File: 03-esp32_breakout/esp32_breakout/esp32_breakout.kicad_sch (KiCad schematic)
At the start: 0 parts

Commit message: schematic draft
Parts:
- added AE1: Antenna_Chip, wsg_fp:XDCR_2450AT18B100E, symbol Device:Antenna_Chip
- added C1, C2, C5, C6: 10µF, symbol Device:C
- added C10, C9: 1.5pF, Capacitor_SMD:C_0201_0603Metric, symbol Device:C
- added C11: 1.2pF, Capacitor_SMD:C_0201_0603Metric, symbol Device:C
- added C3, C4: 0.1µF, symbol Device:C
- added C7, C8: 14µF, symbol Device:C
- added J1: USB4110-GF-A, USB4110-GF-A_GCT, symbol USB4110:USB4110-GF-A
- added J2: Conn_01x16, symbol Connector_Generic:Conn_01x16
- added J3: Conn_01x04, symbol Connector_Generic:Conn_01x04
- added J4: Conn_01x02, symbol Connector_Generic:Conn_01x02
- added J5: Conn_01x06, symbol Connector_Generic:Conn_01x06
- added L1: 2.2nH, symbol Device:L
- added L2: 2.7nH, Inductor_SMD:L_0201_0603Metric, symbol Device:L
- added L3: 3.3nH, Inductor_SMD:L_0402_1005Metric, symbol Device:L
- added L4: 2.7nH, Inductor_SMD:L_0402_1005Metric, symbol Device:L
- added R1, R2, R5: 10k, Resistor_SMD:R_0402_1005Metric, symbol Device:R
- added R3, R4: 5.1k, Resistor_SMD:R_0402_1005Metric, symbol Device:R
- added SW1, SW2: SW_Push, symbol Switch:SW_Push
- added U1: ESP32-S3, Package_DFN_QFN:QFN-56-1EP_7x7mm_P0.4mm_EP4x4mm, symbol MCU_Espressif:ESP32-S3
- added U2: USBLC6-2SC6, USBLC6-2SC6:SOT95P280X145-6N, symbol USB4110:USBLC6-2SC6
- added U3: AP2112K-3.3, Package_TO_SOT_SMD:SOT-23-5, symbol Regulator_Linear:AP2112K-3.3
- added Y1: ECS-400-10-37B2-CKY-TR, ECS-400-10-37B2-CKY-TR:XTAL_ECS-400-10-37B2-CKY-TR, symbol USB4110:ECS-400-10-37B2-CKY-TR
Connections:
- new net: R2.1, SW2.1, U1.4 (CHIP_PU)
- new net: C9.2, L2.1, U1.1 (LNA_IN)
- new net: J2.12 (Pin_12), U1.10 (GPIO5)
- new net: J2.11 (Pin_11), U1.11 (GPIO6)
- new net: J2.10 (Pin_10), U1.12 (GPIO7)
- new net: J2.9 (Pin_9), U1.13 (GPIO8)
- new net: J2.8 (Pin_8), U1.14 (GPIO9)
- new net: J2.7 (Pin_7), U1.15 (GPIO10)
- new net: J2.6 (Pin_6), U1.16 (GPIO11)
- new net: J2.5 (Pin_5), U1.17 (GPIO12)
- new net: J2.4 (Pin_4), U1.18 (GPIO13)
- new net: J2.3 (Pin_3), U1.19 (GPIO14)
- new net: C4.2, L1.2, U1.2 (VDD3P3), U1.3 (VDD3P3)
- new net: J2.2 (Pin_2), U1.23 (GPIO17)
- new net: J2.1 (Pin_1), U1.24 (GPIO18)
- new net: U1.25 (GPIO19/USB_D-), U2.6
- new net: U1.26 (GPIO20/USB_D+), U2.4
- new net: J5.1 (Pin_1), U1.39 (GPIO34)
- new net: J5.2 (Pin_2), U1.40 (GPIO35)
- new net: J5.3 (Pin_3), U1.41 (GPIO36)
- new net: J5.4 (Pin_4), U1.42 (GPIO37)
- new net: J5.5 (Pin_5), U1.43 (GPIO38)
- new net: J5.6 (Pin_6), U1.44 (MTCK)
- new net: J4.1 (Pin_1), U1.49 (U0TXD)
- new net: R1.2, SW1.1, U1.5 (GPIO0)
- new net: J4.2 (Pin_2), U1.50 (U0RXD)
- new net: R5.1, U1.51 (GPIO45), U1.52 (GPIO46)
- new net: C7.2, U1.53 (XTAL_N), Y1.3
- new net: C8.2, U1.54 (XTAL_P), Y1.1
- new net: J2.16 (Pin_16), U1.6 (GPIO1)
- new net: J2.15 (Pin_15), U1.7 (GPIO2)
- new net: J2.14 (Pin_14), U1.8 (GPIO3)
- new net: J2.13 (Pin_13), U1.9 (GPIO4)
- new net: J1.A4-B9 (VBUS), J3.2 (Pin_2)
- new net: J1.A5 (CC1), R4.1
- new net: J1.B5 (CC2), R3.1
- new net: C11.1, L3.1, L4.2
- new net: AE1.1 (FEED), L3.2
- new net: C10.2, C11.2, L2.2
- new net 3v3: C2.2, C3.2, C5.2, C6.2, J3.1 (Pin_1), L1.1, R2.2, U1.20 (VDD3P3_RTC), U1.29 (VDD_SPI), U1.46 (VDD3P3_CPU), U1.55 (VDDA), U1.56 (VDDA), U3.5 (VOUT)
- new net 5v_USB_EXT: C1.2, J1.A9-B4 (VBUS), U2.2, U3.1 (VIN), U3.3 (EN)
- new net GND: J3.3 (Pin_3), J3.4 (Pin_4)
- new net GNDA: AE1.2 (PCB_Trace), C10.1, C9.1, L4.1
- new net GNDD: C1.1, C2.1, C3.1, C4.1, C5.1, C6.1, C7.1, C8.1, J1.A1-B12 (GND), J1.A12-B1 (GND), R1.1, R3.2, R4.2, R5.2, SW1.2, SW2.2, U1.57 (GND), U2.5, U3.2 (GND), Y1.2, Y1.4
- new net RTC?: U1.21 (XTAL_32K_P), U1.22 (XTAL_32K_N)
- new net USB_D+_EXT: J1.A6 (DP1), J1.B7 (DN2), U2.3
- new net USB_D-_EXT: J1.A7 (DN1), J1.B6 (DP2), U2.1
- no-connect marks 0 -> 2

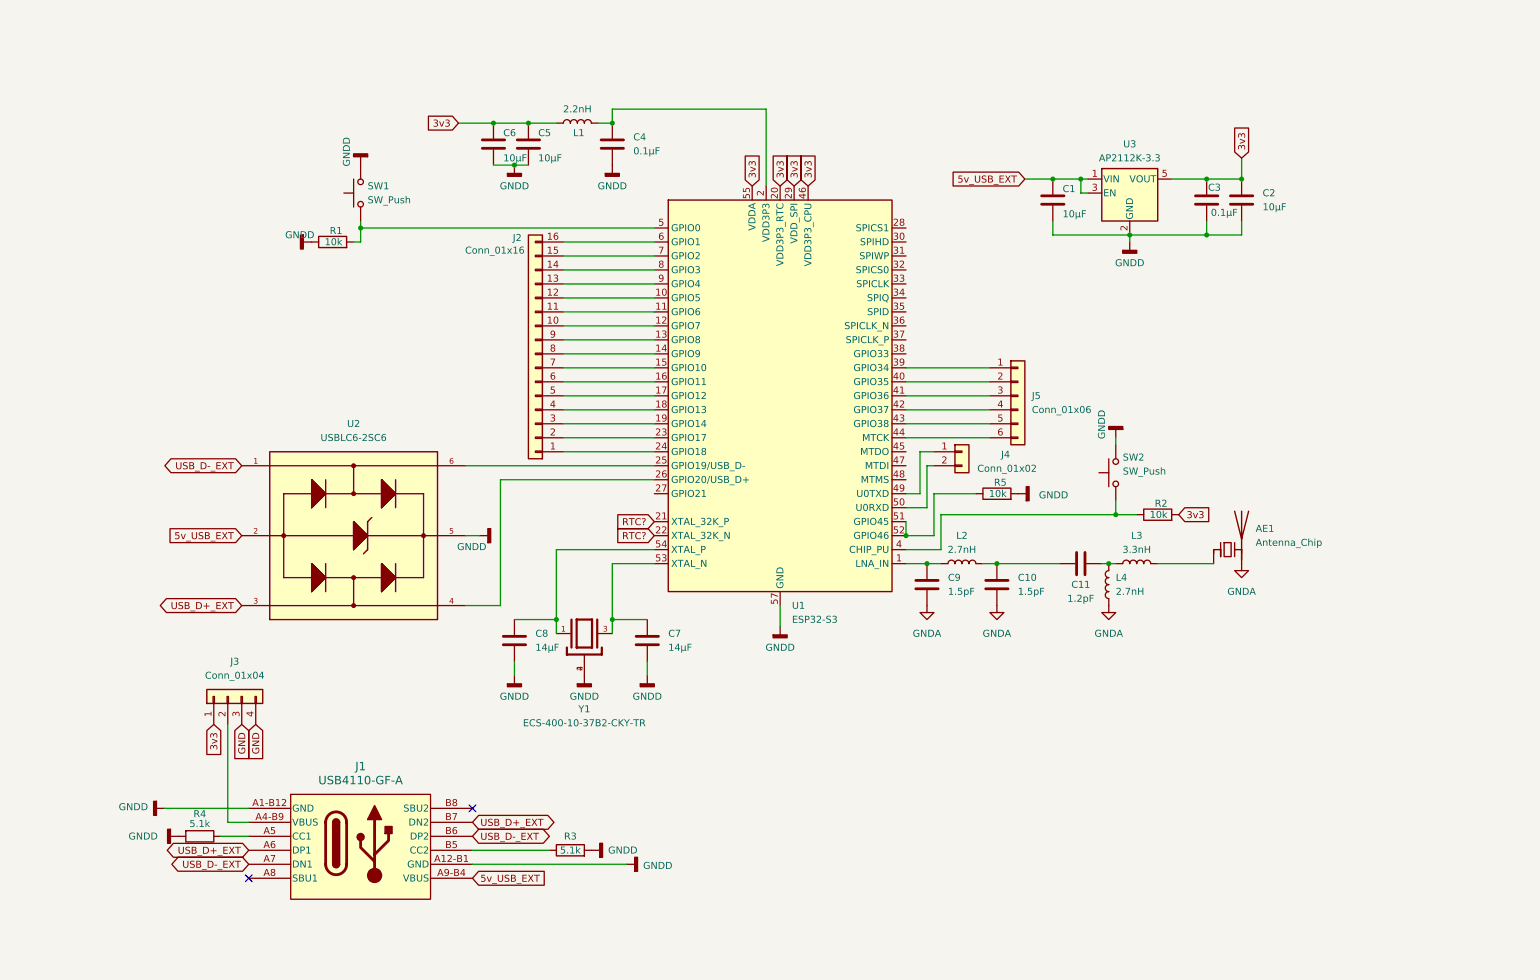
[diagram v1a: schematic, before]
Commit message: first schematic draft
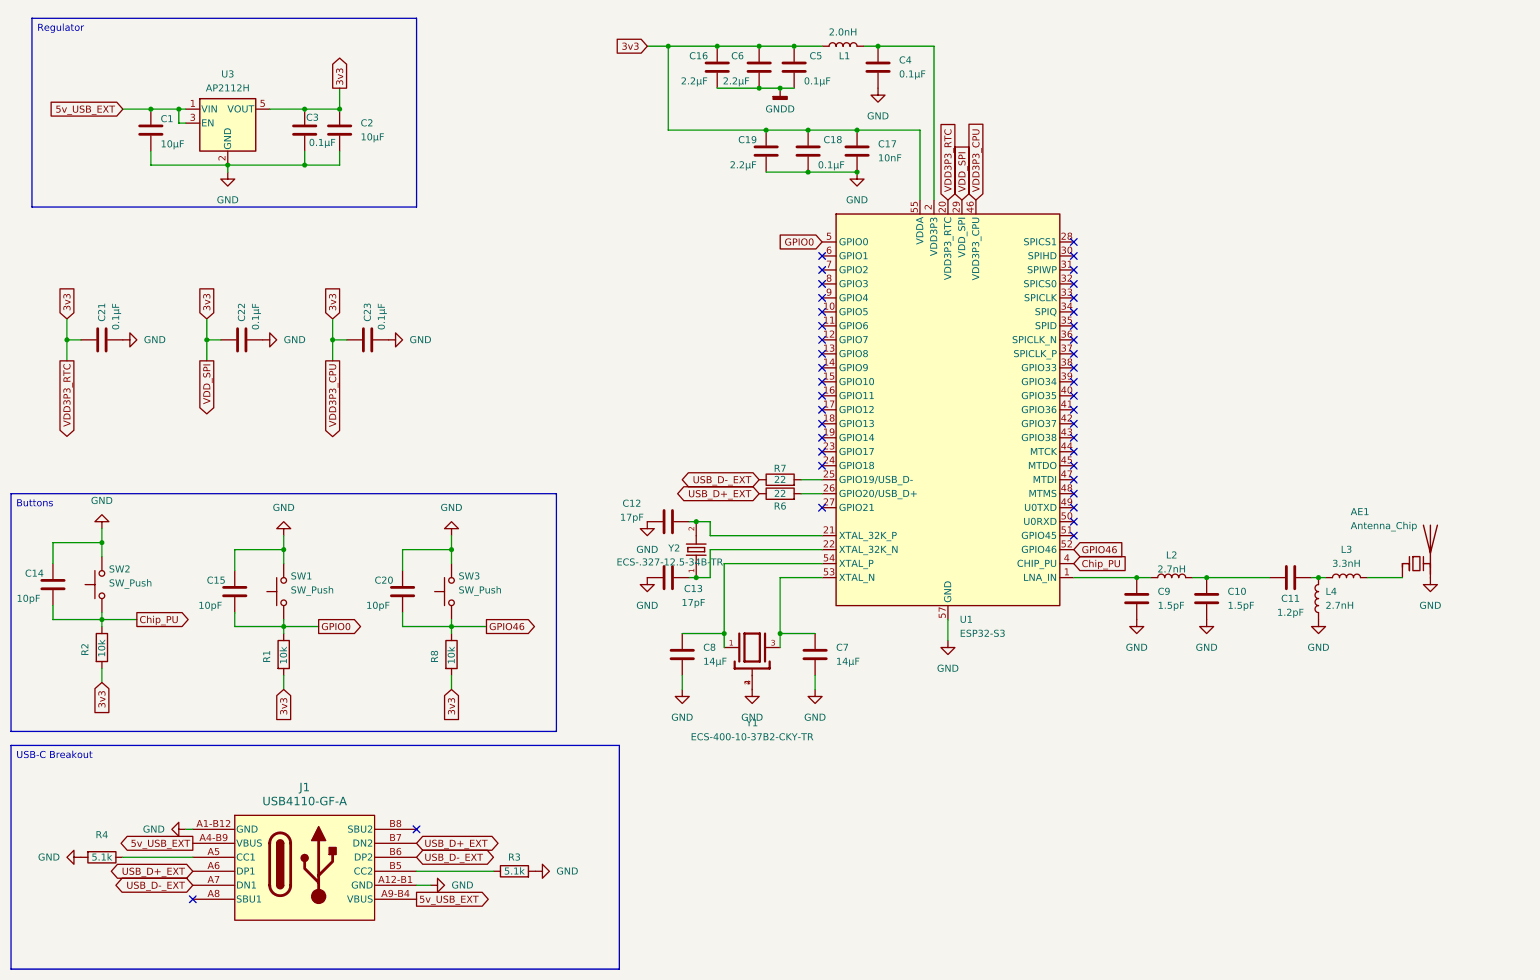
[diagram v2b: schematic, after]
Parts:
- removed J2: Conn_01x16, symbol Connector_Generic:Conn_01x16
- removed J3: Conn_01x04, symbol Connector_Generic:Conn_01x04
- removed J4: Conn_01x02, symbol Connector_Generic:Conn_01x02
- removed J5: Conn_01x06, symbol Connector_Generic:Conn_01x06
- removed R5: 10k, Resistor_SMD:R_0402_1005Metric, symbol Device:R
- removed U2: USBLC6-2SC6, USBLC6-2SC6:SOT95P280X145-6N, symbol USB4110:USBLC6-2SC6
- added C12, C13: 17pF, Capacitor_SMD:C_0402_1005Metric, symbol Device:C
- added C14, C15, C20: 10pF, Capacitor_SMD:C_0402_1005Metric, symbol Device:C
- added C16, C19: 2.2µF, Capacitor_SMD:C_0402_1005Metric, symbol Device:C
- added C17: 10nF, Capacitor_SMD:C_0402_1005Metric, symbol Device:C
- added C18, C21, C22, C23: 0.1µF, Capacitor_SMD:C_0402_1005Metric, symbol Device:C
- added R6, R7: 22, Resistor_SMD:R_0402_1005Metric, symbol Device:R
- added R8: 10k, Resistor_SMD:R_0402_1005Metric, symbol Device:R
- added SW3: SW_Push, symbol Switch:SW_Push
- added Y2: ECS-.327-12.5-34B-TR, wsg_fp:XTAL_ECS-.327-12.5-34B-TR, symbol wsg_syms:ECS-.327-12.5-34B-TR
- C1, C2, C3, C4, C7, C8: footprint (none) -> Capacitor_SMD:C_0402_1005Metric
- C5: value 10µF -> 0.1µF; footprint (none) -> Capacitor_SMD:C_0402_1005Metric
- C6: value 10µF -> 2.2µF; footprint (none) -> Capacitor_SMD:C_0402_1005Metric
- L1: value 2.2nH -> 2.0nH
- U3: value AP2112K-3.3 -> AP2112H
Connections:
- net GNDA is gone; now on net GND: AE1.2 (PCB_Trace), C10.1, C9.1, L4.1
- net 5v_USB_EXT: now also J1.A4-B9 (VBUS)
- net GND: now also C1.1, C2.1, C3.1, C4.1, C7.1, C8.1, J1.A1-B12 (GND), J1.A12-B1 (GND), R3.2, R4.2, SW1.2, SW2.2, U1.57 (GND), U3.2 (GND), Y1.2, Y1.4, C12.1, C13.2, C14.2, C15.2, C17.1, C18.1, C19.1, C20.2, C21.1, C22.1, C23.1, SW3.2
- net GNDD: now also C16.1; no longer C1.1, C2.1, C3.1, C4.1, C7.1, C8.1, J1.A1-B12 (GND), J1.A12-B1 (GND), R1.1, R3.2, R4.2, SW1.2, SW2.2, U1.57 (GND), U3.2 (GND), Y1.2, Y1.4
- net USB_D+_EXT: now also R6.1
- net USB_D-_EXT: now also R7.1
- net Chip_PU: now reaches R2.1, SW2.1, U1.4 (CHIP_PU)
- net Chip_PU: now also C14.1
- net at U1.25 (GPIO19/USB_D-): now also R7.2
- net at U1.26 (GPIO20/USB_D+): now also R6.2
- net GPIO0: now reaches SW1.1, U1.5 (GPIO0)
- net GPIO0: now also R1.1, C15.1; no longer R1.2
- net at U1.51 (GPIO45): no longer U1.52 (GPIO46)
- net 3v3 renamed  VDD3P3_RTC
- net  VDD3P3_RTC: now also R1.2, C16.2, C17.2, C18.2, C19.2, C21.2, C22.2, C23.2, R8.2
- net RTC?: no longer names the net of U1.21 (XTAL_32K_P)
- net RTC?: now also C12.2, Y2.2; no longer U1.22 (XTAL_32K_N)
- new net: C13.1, U1.22 (XTAL_32K_N), Y2.1
- new net GPIO46: C20.1, R8.1, SW3.1, U1.52 (GPIO46)
- no-connect marks 2 -> 41
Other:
- moved on the sheet: AE1, C1, C10, C11, C2, C3, C4, C5, C6, C7, C8, C9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

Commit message: layout first draft
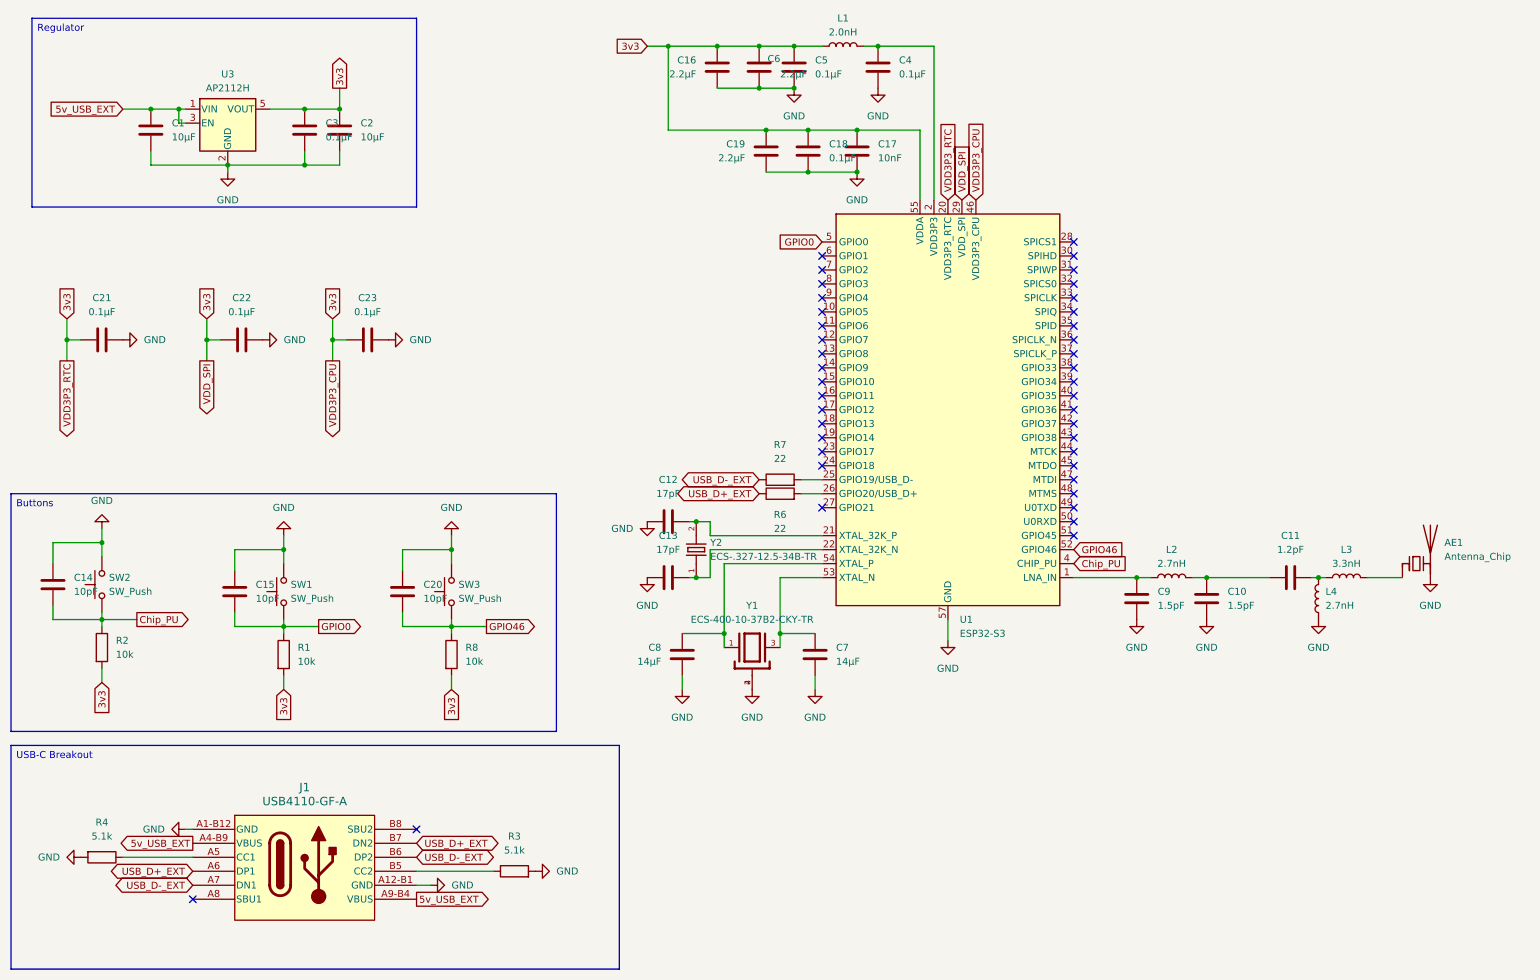
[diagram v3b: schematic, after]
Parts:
- J1: footprint USB4110-GF-A_GCT -> wsg_fp:USB4110-GF-A_GCT
- L1: footprint (none) -> Inductor_SMD:L_0402_1005Metric
- SW1, SW2, SW3: footprint (none) -> wsg_fp:SW_BUTT-2
- Y1: footprint ECS-400-10-37B2-CKY-TR:XTAL_ECS-400-10-37B2-CKY-TR -> wsg_fp:XTAL_ECS-400-10-37B2-CKY-TR
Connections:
- net GNDD is gone; now on net GND: C16.1, C5.1, C6.1

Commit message: schematics update
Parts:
- SW1, SW2, SW3: footprint wsg_fp:SW_BUTT-2 -> wsg_fp:NANOT100AS_butt
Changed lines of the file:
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@@
 			)
 		)
-		(property "Footprint" "wsg_fp:SW_BUTT-2"
+		(property "Footprint" "wsg_fp:NANOT100AS_butt"
 			(at 27.94 121.92 0)
 			(effects
@@
 			)
 		)
-		(property "Footprint" "wsg_fp:SW_BUTT-2"
+		(property "Footprint" "wsg_fp:NANOT100AS_butt"
 			(at 91.44 123.19 0)
 			(effects
@@
 			)
 		)
-		(property "Footprint" "wsg_fp:SW_BUTT-2"
+		(property "Footprint" "wsg_fp:NANOT100AS_butt"
 			(at 60.96 123.19 0)
 			(effects
